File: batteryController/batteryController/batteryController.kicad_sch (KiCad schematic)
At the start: 15 parts, among them J1 Conn_01x02_Male, J2 Screw_Terminal_01x02, J3 Conn_01x04_Male, J4 Conn_01x04_Male, J5 Conn_01x04_Male, J6 USB_A, U1 ATtiny13V-10P, U2 L7806CV, U3 L78L05_TO92

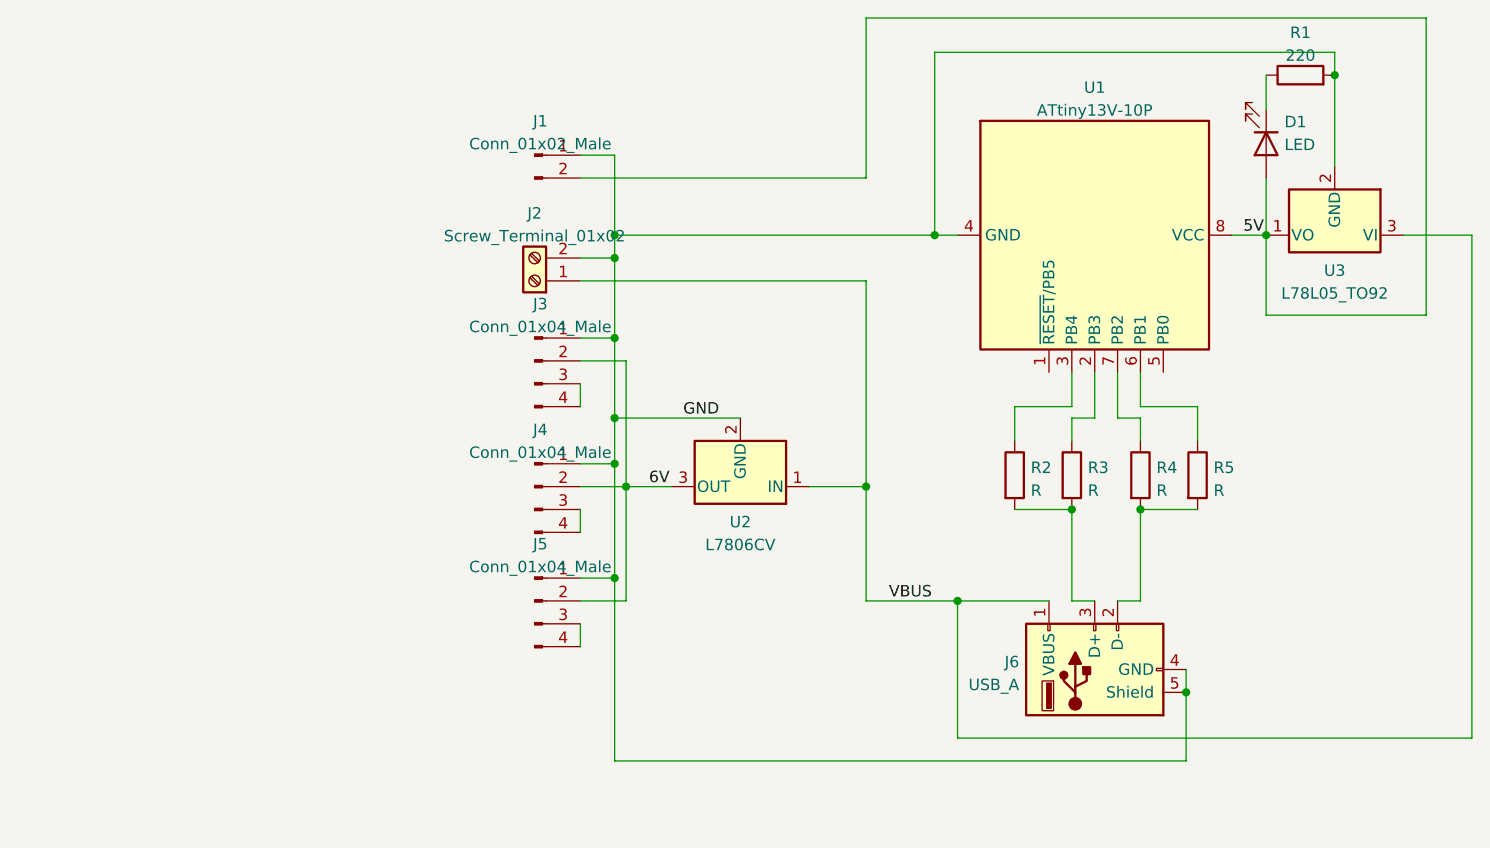
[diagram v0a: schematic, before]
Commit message: remade basically the entire thing
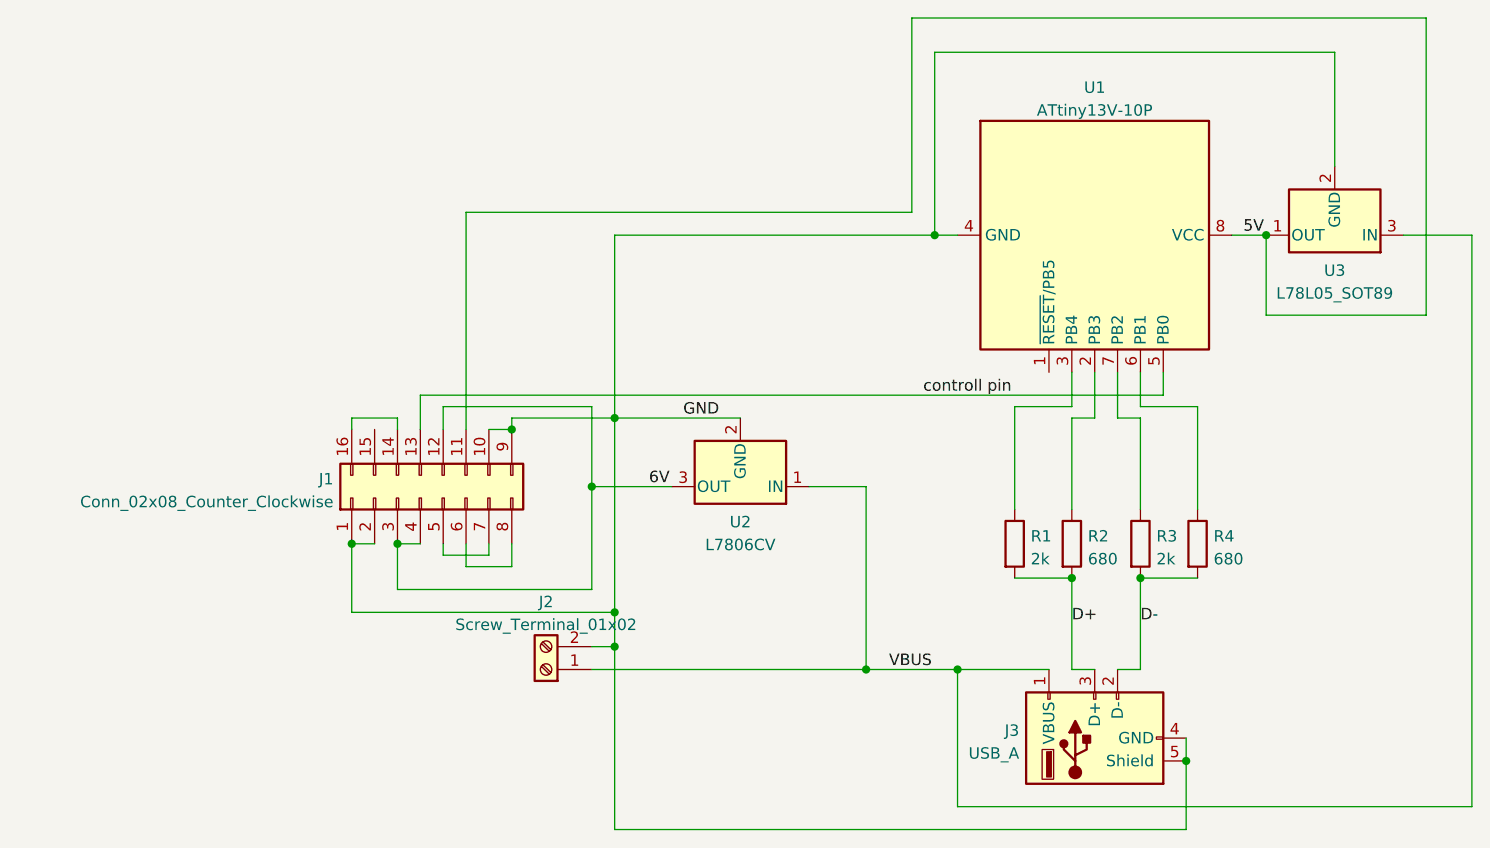
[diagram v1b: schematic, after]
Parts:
- removed D1: LED, LED_THT:LED_D3.0mm, symbol Device:LED
- removed J1: Conn_01x02_Male, Connector_PinHeader_2.54mm:PinHeader_1x02_P2.54mm_Vertical, symbol Connector:Conn_01x02_Male
- removed J3, J4, J5: Conn_01x04_Male, Connector_PinHeader_2.54mm:PinHeader_1x04_P2.54mm_Vertical, symbol Connector:Conn_01x04_Male
- removed R1: 220, Resistor_THT:R_Axial_DIN0207_L6.3mm_D2.5mm_P7.62mm_Horizontal, symbol Device:R
- removed U3: L78L05_TO92, Package_TO_SOT_THT:TO-92_Inline, symbol Regulator_Linear:L78L05_TO92
- added J1: Conn_02x08_Counter_Clockwise, Connector_PinHeader_2.54mm:PinHeader_2x08_P2.54mm_Vertical, symbol Connector_Generic:Conn_02x08_Counter_Clockwise
- added U3: L78L05_SOT89, Package_TO_SOT_SMD:SOT-89-3, symbol Regulator_Linear:L78L05_SOT89
- R1: renamed from R2; value R -> 2k; footprint Resistor_THT:R_Axial_DIN0207_L6.3mm_D2.5mm_P7.62mm_Horizontal -> Resistor_SMD:R_0603_1608Metric
- R2: renamed from R3; value R -> 680; footprint Resistor_THT:R_Axial_DIN0207_L6.3mm_D2.5mm_P7.62mm_Horizontal -> Resistor_SMD:R_0603_1608Metric
- R3: renamed from R4; value R -> 2k; footprint Resistor_THT:R_Axial_DIN0207_L6.3mm_D2.5mm_P7.62mm_Horizontal -> Resistor_SMD:R_0603_1608Metric
- R4: renamed from R5; value R -> 680; footprint Resistor_THT:R_Axial_DIN0207_L6.3mm_D2.5mm_P7.62mm_Horizontal -> Resistor_SMD:R_0603_1608Metric
- renumbered J6 to J3
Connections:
- net 5V: now also J1.11 (Pin_11), U3.1 (OUT)
- net 6V: now also J1.12 (Pin_12), J1.3 (Pin_3), J1.4 (Pin_4)
- net GND: now also J1.1 (Pin_1), J1.10 (Pin_10), J1.2 (Pin_2), J1.9 (Pin_9), U3.2 (GND)
- net VBUS: now also U3.3 (IN)
- net controll pin: now reaches U1.5 (PB0)
- net controll pin: now also J1.13 (Pin_13)
- net D-: now reaches J3.2 (D-), R3.2, R4.2
- net D+: now reaches J3.3 (D+), R1.2, R2.2
- new net: J1.14 (Pin_14), J1.16 (Pin_16)
- new net: J1.5 (Pin_5), J1.7 (Pin_7)
- new net: J1.6 (Pin_6), J1.8 (Pin_8)
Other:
- moved on the sheet: J2, J3, R1, R2, R3, R4
